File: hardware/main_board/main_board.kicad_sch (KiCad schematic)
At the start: 0 parts

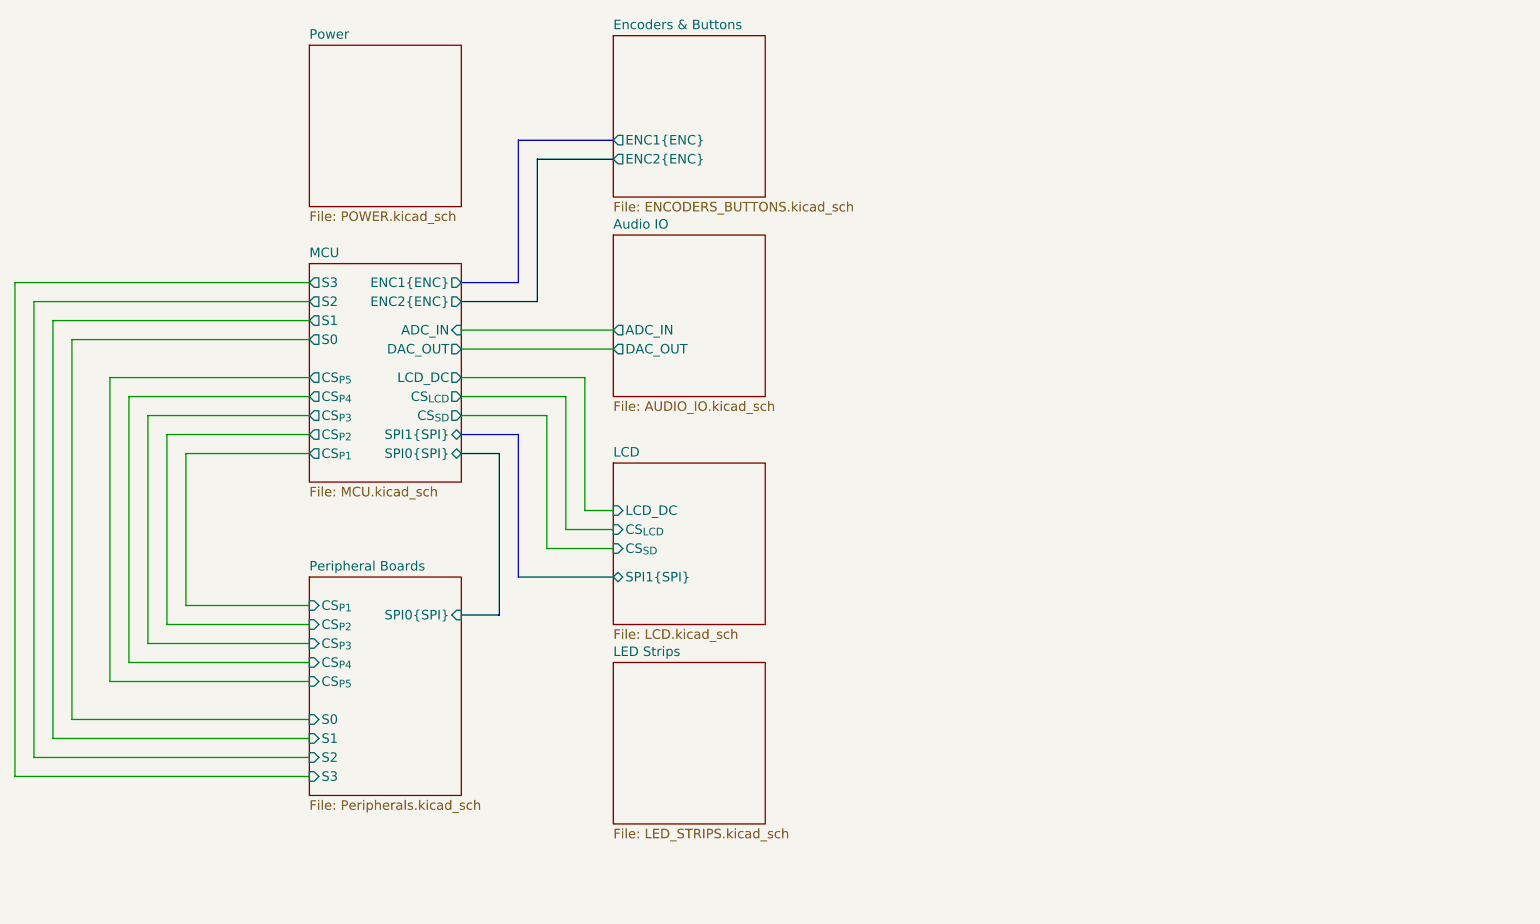
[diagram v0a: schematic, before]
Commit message: save before nuke SPI ADC
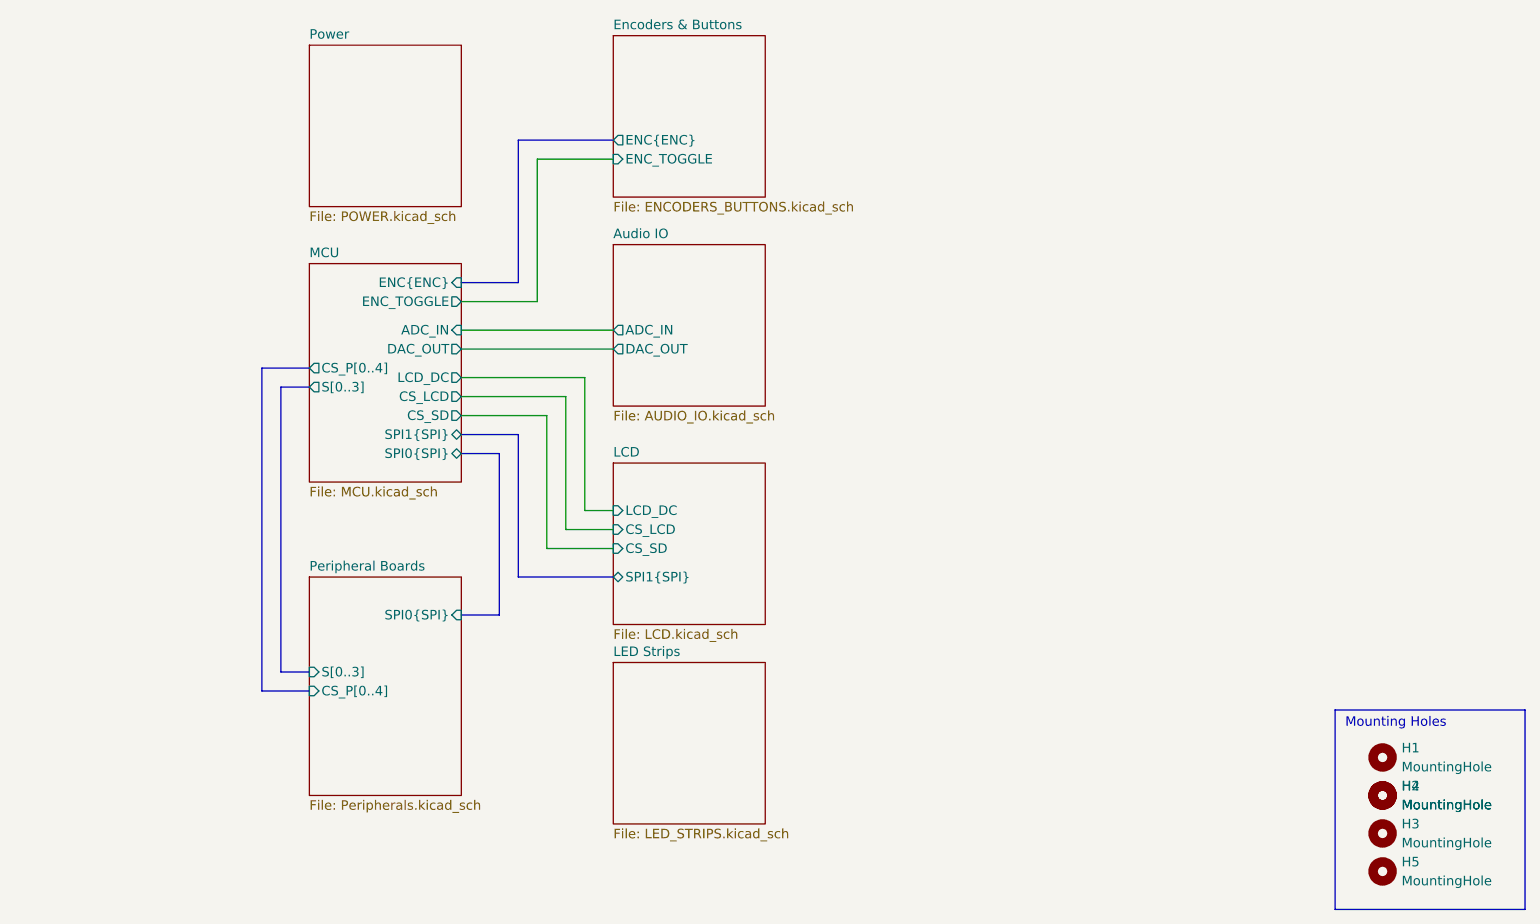
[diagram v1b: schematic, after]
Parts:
- added H1, H2, H3, H4, H5: MountingHole, symbol Mechanical:MountingHole
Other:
- sheet Encoders & Buttons ports: added ENC_TOGGLE, ENC{ENC}; removed ENC1{ENC}, ENC2{ENC}
- sheet LCD ports: added CS_LCD, CS_SD; removed CS_{LCD}, CS_{SD}
- sheet MCU ports: added CS_LCD, CS_P[0..4], CS_SD, ENC_TOGGLE, ENC{ENC}, S[0..3]; removed CS_{LCD}, CS_{P1}, CS_{P2}, CS_{P3}, CS_{P4}, CS_{P5}, CS_{SD}, ENC1{ENC}, ENC2{ENC}, S0, S1, S2, S3
- sheet Peripheral Boards ports: added CS_P[0..4], S[0..3]; removed CS_{P1}, CS_{P2}, CS_{P3}, CS_{P4}, CS_{P5}, S0, S1, S2, S3
- note added: "Mounting Holes"
